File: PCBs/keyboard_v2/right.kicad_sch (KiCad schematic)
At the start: 0 parts

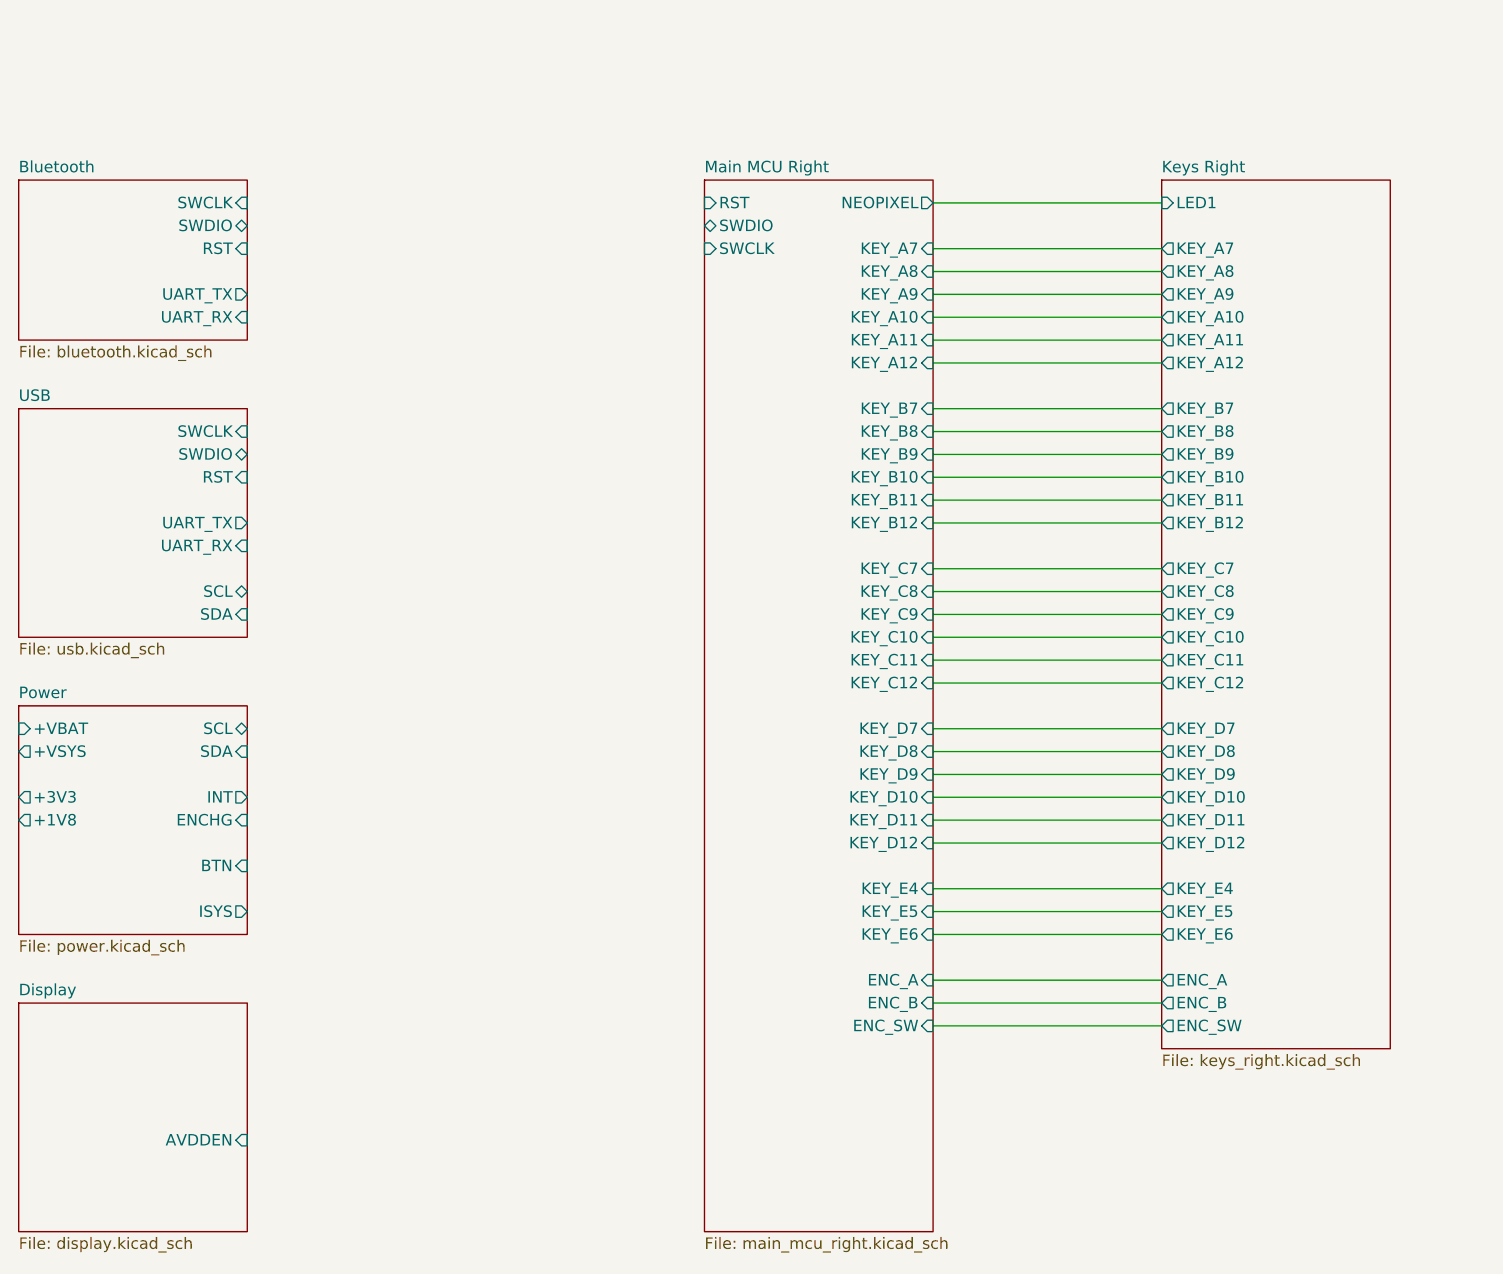
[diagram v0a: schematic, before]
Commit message: V2 Progress
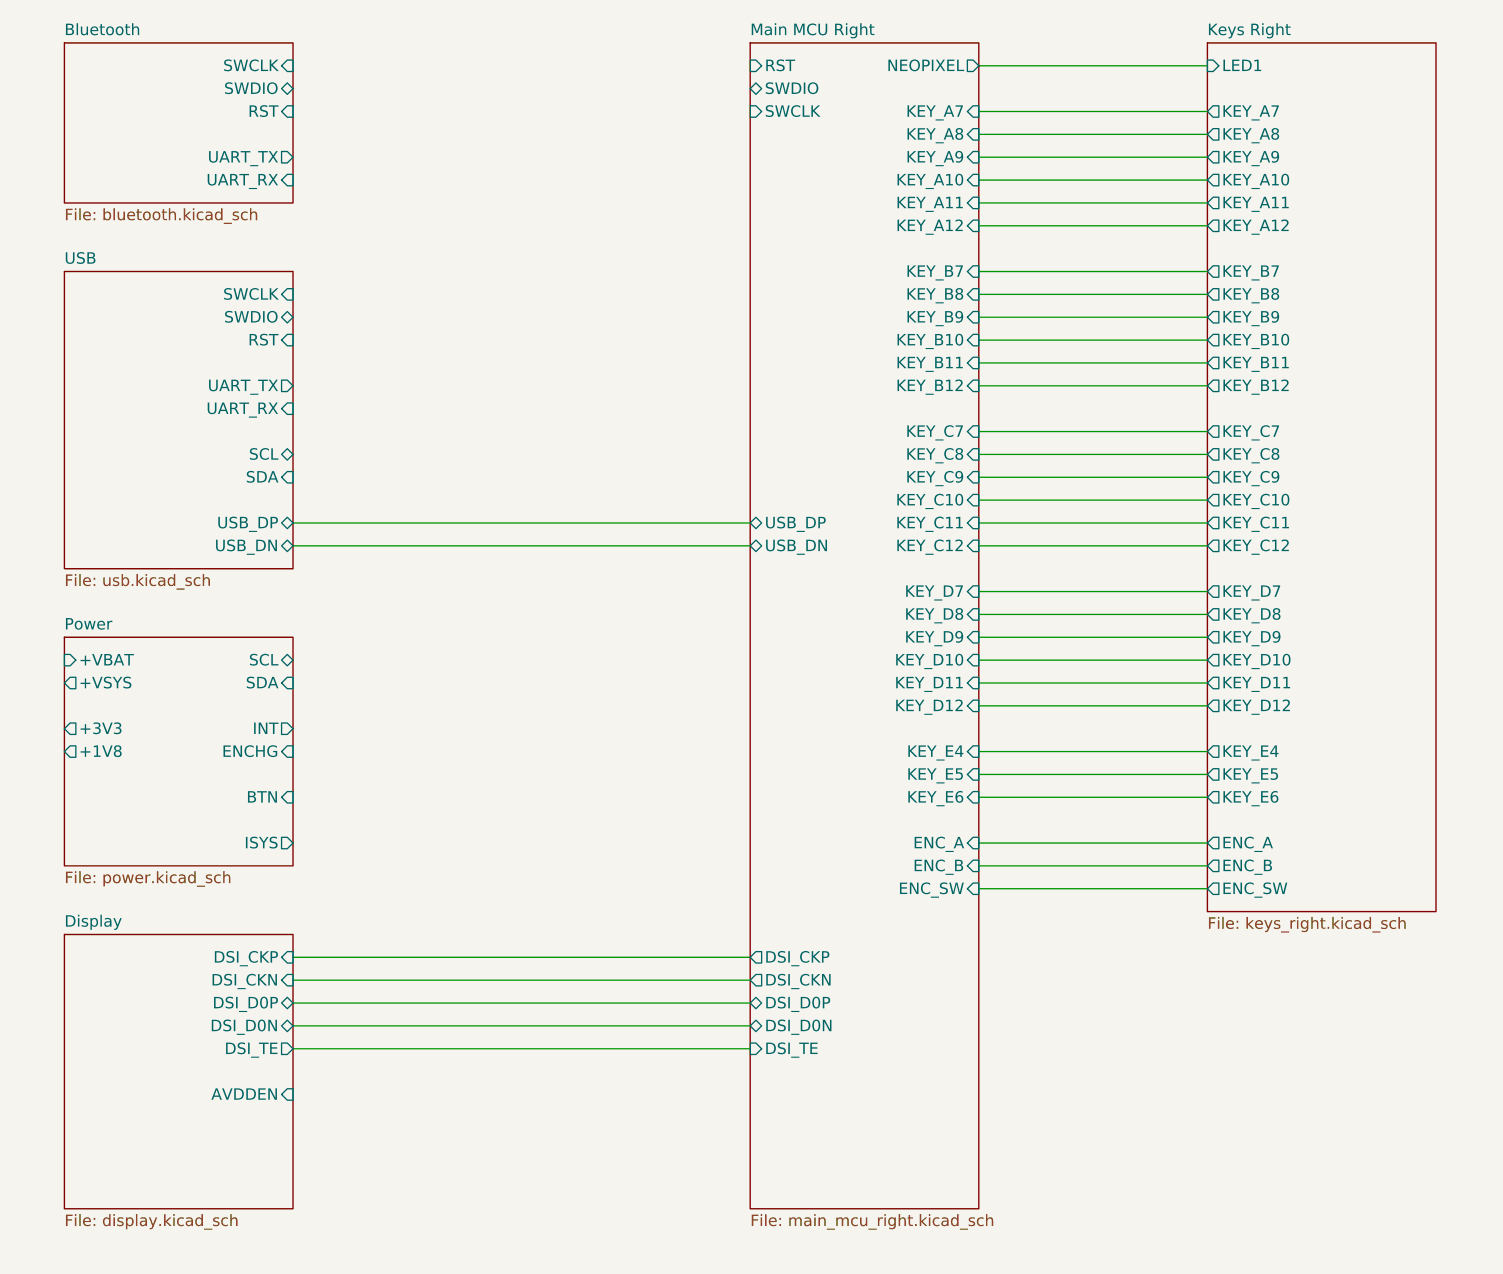
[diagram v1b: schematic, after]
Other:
- sheet Display ports: added DSI_CKN, DSI_CKP, DSI_D0N, DSI_D0P, DSI_TE; removed none
- sheet Main MCU Right ports: added DSI_CKN, DSI_CKP, DSI_D0N, DSI_D0P, DSI_TE, USB_DN, USB_DP; removed none
- sheet USB ports: added USB_DN, USB_DP; removed none
